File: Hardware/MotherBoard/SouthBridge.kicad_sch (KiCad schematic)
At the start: 12 parts, among them J12 NMI_PULLUP, J14 IRQ0_PULLUP, J3 ISA1, J4 ISA0, U10 74HC245, U11 74HC245, U12 74HC245, U13 74HC541, U14 74HC541, U9 74HC245

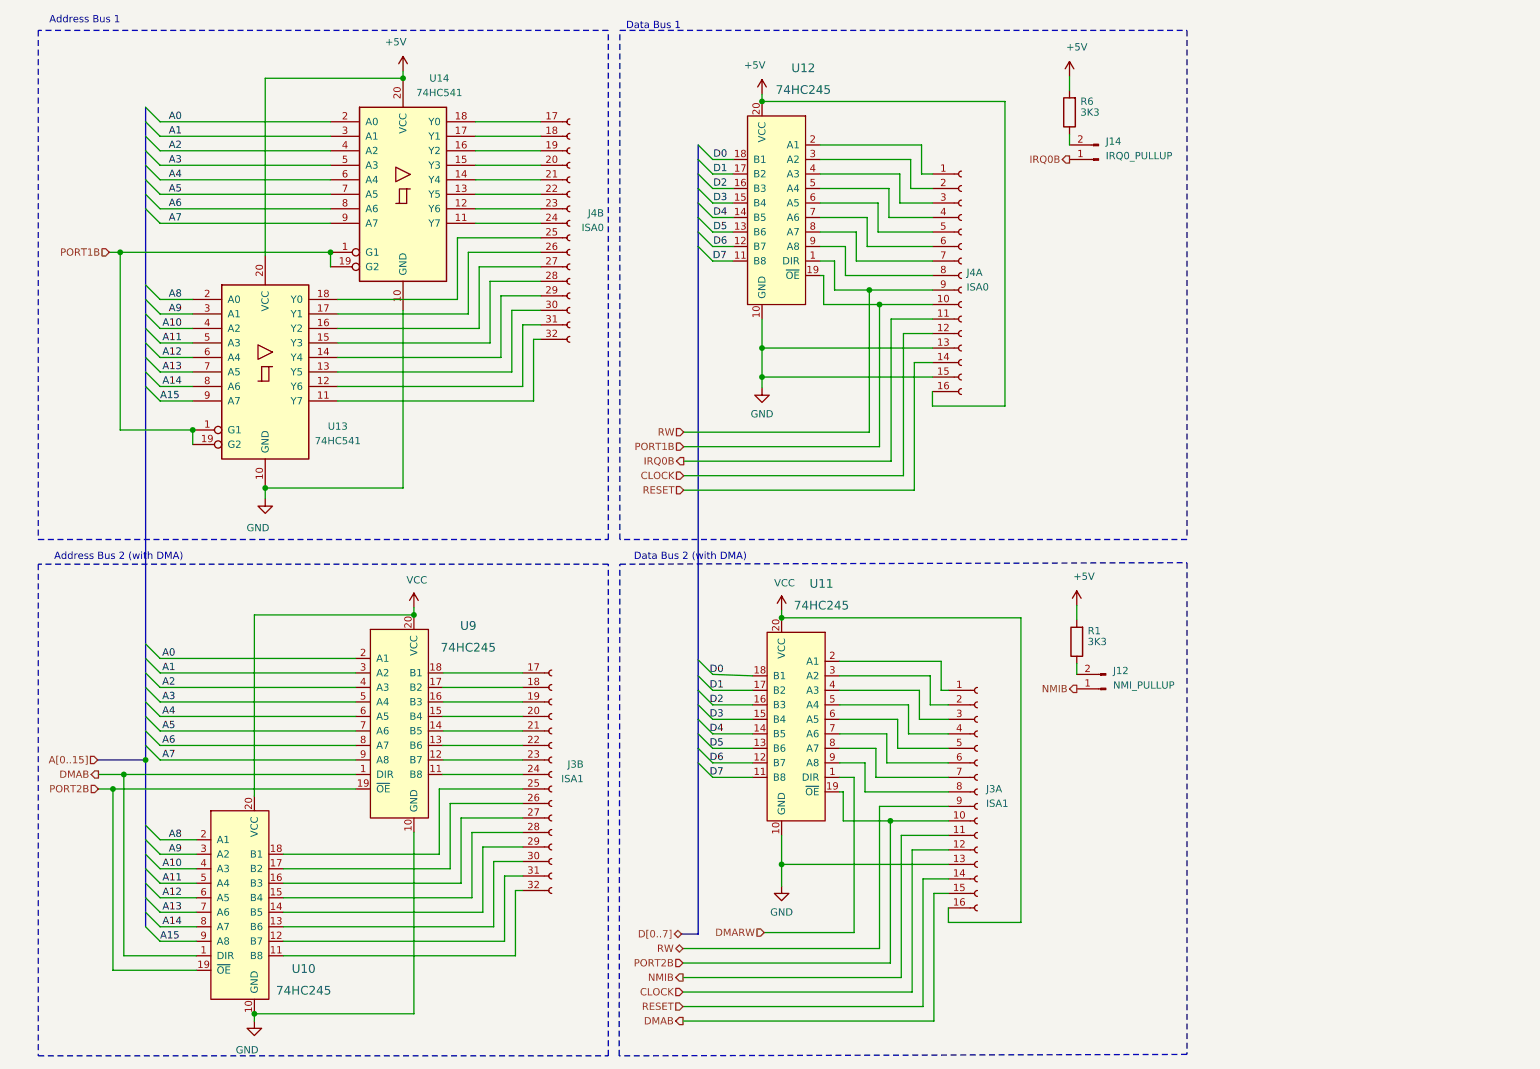
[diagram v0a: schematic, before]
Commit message: New motherboard version
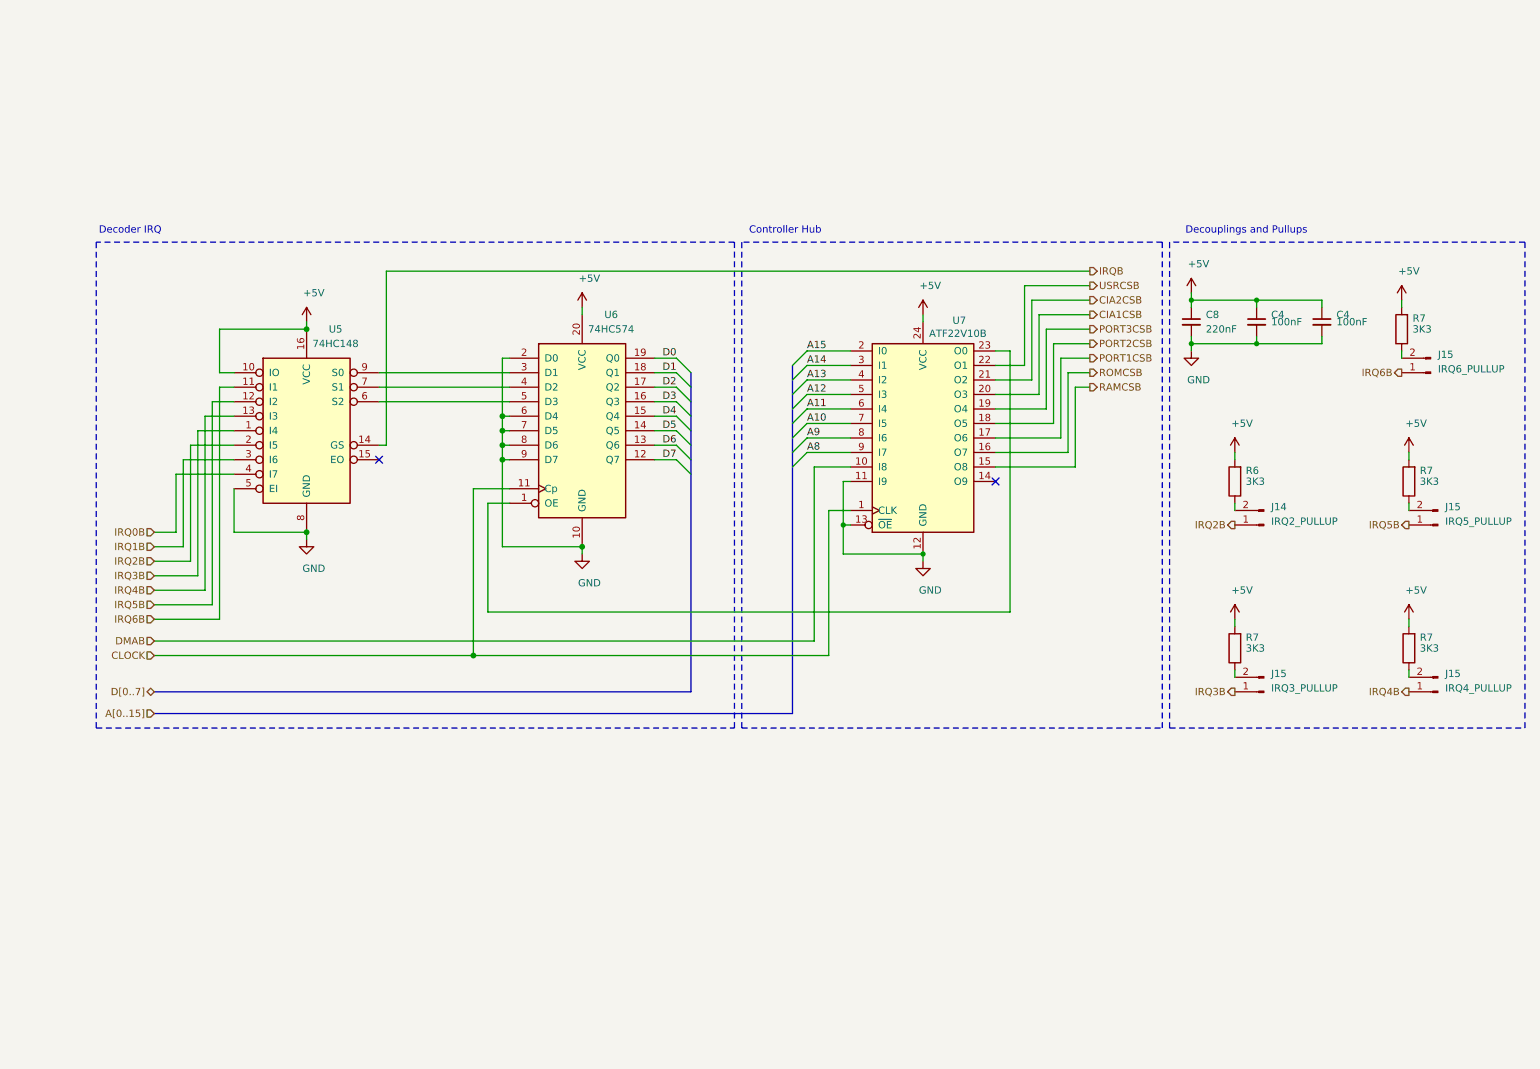
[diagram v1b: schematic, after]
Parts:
- removed J12: NMI_PULLUP, Connector_PinHeader_2.54mm:PinHeader_1x02_P2.54mm_Vertical, symbol Connector:Conn_01x02_Male
- removed J14: IRQ0_PULLUP, Connector_PinHeader_2.54mm:PinHeader_1x02_P2.54mm_Vertical, symbol Connector:Conn_01x02_Male
- removed J3: ISA1, Connector_PinSocket_2.54mm:PinSocket_2x16_P2.54mm_Vertical, symbol Connector_TheRLab:Conn_02x16_Female_2units
- removed J4: ISA0, Connector_PinSocket_2.54mm:PinSocket_2x16_P2.54mm_Vertical, symbol Connector_TheRLab:Conn_02x16_Female_2units
- removed R1: 3K3, Resistor_THT:R_Axial_DIN0207_L6.3mm_D2.5mm_P10.16mm_Horizontal, symbol Device:R
- removed U10, U11, U12, U9: 74HC245, Package_DIP:DIP-20_W7.62mm, symbol dk_Logic-Buffers-Drivers-Receivers-Transceivers:SN74LVC245AN
- removed U13, U14: 74HC541, Package_DIP:DIP-20_W7.62mm, symbol 74xx:74HCT541
- added C4 (x2): 100nF, Capacitor_THT:C_Disc_D5.0mm_W2.5mm_P2.50mm, symbol Device:C_Small
- added C8: 220nF, Capacitor_THT:C_Disc_D5.0mm_W2.5mm_P5.00mm, symbol Device:C_Small
- added J14: IRQ2_PULLUP, Connector_PinHeader_2.54mm:PinHeader_1x02_P2.54mm_Vertical, symbol Connector:Conn_01x02_Pin
- added J15: IRQ5_PULLUP, Connector_PinHeader_2.54mm:PinHeader_1x02_P2.54mm_Vertical, symbol Connector:Conn_01x02_Pin
- added J15: IRQ4_PULLUP, Connector_PinHeader_2.54mm:PinHeader_1x02_P2.54mm_Vertical, symbol Connector:Conn_01x02_Pin
- added J15: IRQ3_PULLUP, Connector_PinHeader_2.54mm:PinHeader_1x02_P2.54mm_Vertical, symbol Connector:Conn_01x02_Pin
- added J15: IRQ6_PULLUP, Connector_PinHeader_2.54mm:PinHeader_1x02_P2.54mm_Vertical, symbol Connector:Conn_01x02_Pin
- added R7 (x4): 3K3, Resistor_THT:R_Axial_DIN0207_L6.3mm_D2.5mm_P10.16mm_Horizontal, symbol Device:R
- added U5: 74HC148, Package_DIP:DIP-16_W7.62mm, symbol 74xx:74LS148
- added U6: 74HC574, Package_DIP:DIP-20_W7.62mm, symbol 74xx:74HCT574
- added U7: ATF22V10B, Package_DIP:DIP-24_W7.62mm, symbol Logic_Programmable:PAL20RS10
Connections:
- net +5V: now also C4.1, C4.1, C8.1, R7.2, R7.2, R7.2, R7.2, U5.10 (IO), U5.16 (VCC), U6.20 (VCC), U7.24 (VCC)
- net A10: now also U7.7 (I5)
- net A11: now also U7.6 (I4)
- net A12: now also U7.5 (I3)
- net A13: now also U7.4 (I2)
- net A14: now also U7.3 (I1)
- net A15: now also U7.2 (I0)
- net A8: now also U7.9 (I7)
- net A9: now also U7.8 (I6)
- net CLOCK: now also U6.11 (Cp), U7.1 (CLK)
- net D0: now also U6.19 (Q0)
- net D1: now also U6.18 (Q1)
- net D2: now also U6.17 (Q2)
- net D3: now also U6.16 (Q3)
- net D4: now also U6.15 (Q4)
- net D5: now also U6.14 (Q5)
- net D6: now also U6.13 (Q6)
- net D7: now also U6.12 (Q7)
- net DMAB: now also U7.10 (I8)
- net GND: now also C4.2, C4.2, C8.2, U5.5 (EI), U5.8 (GND), U6.10 (GND), U6.2 (D0), U6.6 (D4), U6.7 (D5), U6.8 (D6), U6.9 (D7), U7.11 (I9), U7.12 (GND), U7.13 (~{OE})
- net IRQ0B: now also U5.4 (I7)
- net at R6.1: now also J14.2 (Pin_2)
- new net: J15.2 (Pin_2), R7.1 (x4)
- new net: U5.6 (S2), U6.5 (D3)
- new net: U5.7 (S1), U6.4 (D2)
- new net: U5.9 (S0), U6.3 (D1)
- new net: U6.1 (OE), U7.23 (O0)
- new net CIA1CSB: U7.20 (O3)
- new net CIA2CSB: U7.21 (O2)
- new net IRQ1B: U5.3 (I6)
- new net IRQ2B: J14.1 (Pin_1), U5.2 (I5)
- new net IRQ3B: J15.1 (Pin_1), U5.1 (I4)
- new net IRQ4B: J15.1 (Pin_1), U5.13 (I3)
- new net IRQ5B: J15.1 (Pin_1), U5.12 (I2)
- new net IRQ6B: J15.1 (Pin_1), U5.11 (I1)
- new net IRQB: U5.14 (GS)
- new net PORT1CSB: U7.17 (O6)
- new net PORT2CSB: U7.18 (O5)
- new net PORT3CSB: U7.19 (O4)
- new net RAMCSB: U7.15 (O8)
- new net ROMCSB: U7.16 (O7)
- new net USRCSB: U7.22 (O1)
- no-connect marks 0 -> 2
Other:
- note added: "Controller Hub"
- note added: "Decoder IRQ"
- note added: "Decouplings and Pullups"
- note removed: "Address Bus 1"
- note removed: "Address Bus 2 (with DMA)"
- note removed: "Data Bus 1"
- note removed: "Data Bus 2 (with DMA)"
